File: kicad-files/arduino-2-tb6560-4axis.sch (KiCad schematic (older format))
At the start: 15 parts, among them J1 DB25_Female_MountingHoles, J2 Conn_01x03_Male, J3 Conn_01x02_Male, J4 Conn_01x02_Male, J5 Conn_01x03_Male, J6 Conn_01x02_Male, J7 Conn_01x03_Male, J8 Conn_01x02_Male, J9 Conn_01x02_Male, Q1 2N3904, SW1 SW_Push, SW2 SW_Push

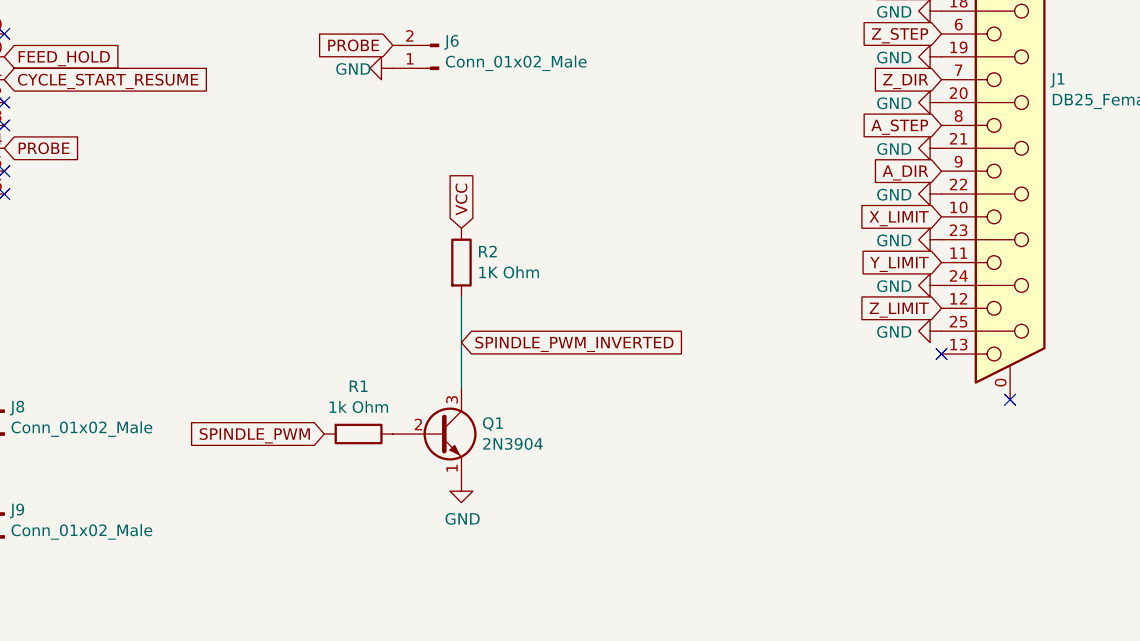
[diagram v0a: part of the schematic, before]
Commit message: more ideas for rev 1.3
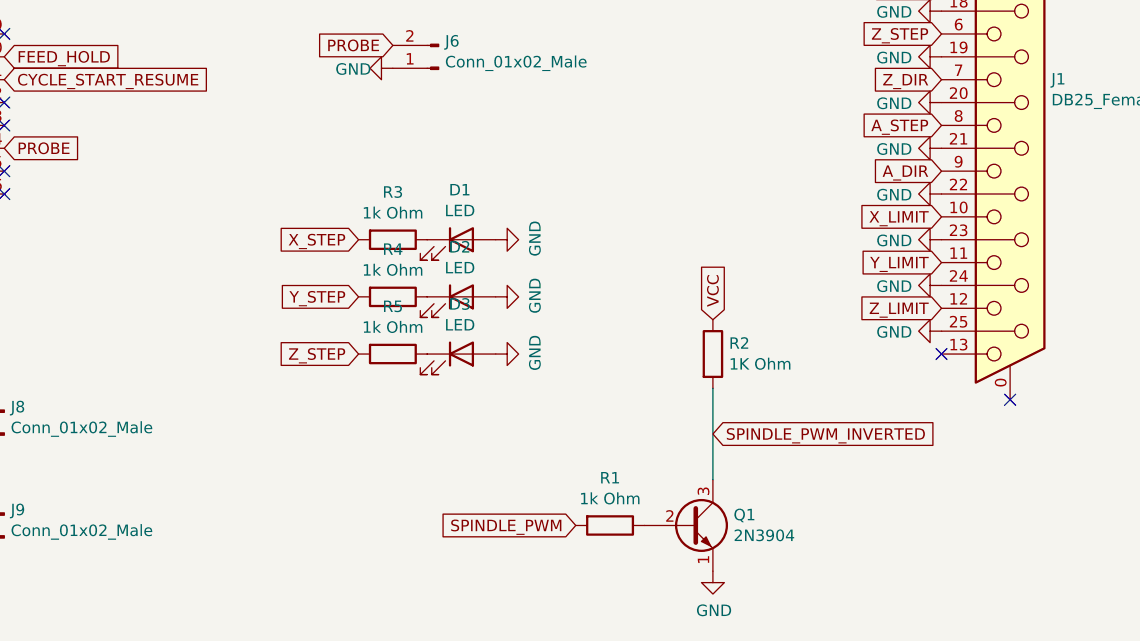
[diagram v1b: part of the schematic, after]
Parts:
- added D1, D2, D3: LED, LED_THT:LED_D5.0mm, symbol Device:LED
- added R3, R4, R5: 1k Ohm, Resistor_THT:R_Axial_DIN0204_L3.6mm_D1.6mm_P5.08mm_Horizontal, symbol Device:R
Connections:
- net GND: now also D1.2 (A), D2.2 (A), D3.2 (A)
- net X_STEP: now also R3.2
- net Y_STEP: now also R4.2
- net Z_STEP: now also R5.2
- new net: D1.1 (K), R3.1
- new net: D2.1 (K), R4.1
- new net: D3.1 (K), R5.1
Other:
- moved on the sheet: Q1, R1, R2
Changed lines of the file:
@@
 L Device:R R1
 U 1 1 5F56F856
-P 5750 5200
-F 0 "R1" V 5543 5200 50  0000 C CNN
-F 1 "1k Ohm" V 5634 5200 50  0000 C CNN
-F 2 "Resistor_THT:R_Axial_DIN0204_L3.6mm_D1.6mm_P5.08mm_Horizontal" V 5680 5200 50  0001 C CNN
-F 3 "~" H 5750 5200 50  0001 C CNN
-	1    5750 5200
+P 6850 5600
+F 0 "R1" V 6643 5600 50  0000 C CNN
+F 1 "1k Ohm" V 6734 5600 50  0000 C CNN
+F 2 "Resistor_THT:R_Axial_DIN0204_L3.6mm_D1.6mm_P5.08mm_Horizontal" V 6780 5600 50  0001 C CNN
+F 3 "~" H 6850 5600 50  0001 C CNN
+	1    6850 5600
 	0    1    1    0
 $EndComp
@@
 L Device:R R2
 U 1 1 5F57191E
-P 6200 4450
-F 0 "R2" H 6270 4496 50  0000 L CNN
-F 1 "1K Ohm" H 6270 4405 50  0000 L CNN
-F 2 "Resistor_THT:R_Axial_DIN0204_L3.6mm_D1.6mm_P5.08mm_Horizontal" V 6130 4450 50  0001 C CNN
-F 3 "~" H 6200 4450 50  0001 C CNN
-	1    6200 4450
+P 7300 4850
+F 0 "R2" H 7370 4896 50  0000 L CNN
+F 1 "1K Ohm" H 7370 4805 50  0000 L CNN
+F 2 "Resistor_THT:R_Axial_DIN0204_L3.6mm_D1.6mm_P5.08mm_Horizontal" V 7230 4850 50  0001 C CNN
+F 3 "~" H 7300 4850 50  0001 C CNN
+	1    7300 4850
 	1    0    0    -1
 $EndComp
@@
 L Transistor_BJT:2N3904 Q1
 U 1 1 5F5721BB
-P 6100 5200
-F 0 "Q1" H 6290 5246 50  0000 L CNN
-F 1 "2N3904" H 6290 5155 50  0000 L CNN
-F 2 "Package_TO_SOT_THT:TO-92_Inline" H 6300 5125 50  0001 L CIN
-F 3 "https://www.fairchildsemi.com/datasheets/2N/2N3904.pdf" H 6100 5200 50  0001 L CNN
-	1    6100 5200
+P 7200 5600
+F 0 "Q1" H 7390 5646 50  0000 L CNN
+F 1 "2N3904" H 7390 5555 50  0000 L CNN
+F 2 "Package_TO_SOT_THT:TO-92_Inline" H 7400 5525 50  0001 L CIN
+F 3 "https://www.fairchildsemi.com/datasheets/2N/2N3904.pdf" H 7200 5600 50  0001 L CNN
+	1    7200 5600
 	1    0    0    -1
 $EndComp
 Text GLabel 3900 2450 1    50   Input ~ 0
 VCC
-Text GLabel 6200 4300 1    50   Input ~ 0
+Text GLabel 7300 4700 1    50   Input ~ 0
 VCC
-Text GLabel 5600 5200 0    50   Input ~ 0
+Text GLabel 6700 5600 0    50   Input ~ 0
 SPINDLE_PWM
 $Comp
 L power:GND #PWR0101
 U 1 1 5F581B0A
-P 6200 5400
-F 0 "#PWR0101" H 6200 5150 50  0001 C CNN
-F 1 "GND" H 6205 5227 50  0000 C CNN
-F 2 "" H 6200 5400 50  0001 C CNN
-F 3 "" H 6200 5400 50  0001 C CNN
-	1    6200 5400
+P 7300 5800
+F 0 "#PWR0101" H 7300 5550 50  0001 C CNN
+F 1 "GND" H 7305 5627 50  0000 C CNN
+F 2 "" H 7300 5800 50  0001 C CNN
+F 3 "" H 7300 5800 50  0001 C CNN
+	1    7300 5800
 	1    0    0    -1
 $EndComp
 Wire Wire Line
-	6200 5000 6200 4600
-Text GLabel 6200 4800 2    50   Input ~ 0
+	7300 5400 7300 5000
+Text GLabel 7300 5200 2    50   Input ~ 0
 SPINDLE_PWM_INVERTED
 Text GLabel 4200 3950 2    50   Input ~ 0
@@
 Text GLabel 4000 5550 0    50   Input ~ 0
 CYCLE_START_RESUME
+$Comp
+L Device:R R3
+U 1 1 5F5D16E5
+P 5900 4350
+F 0 "R3" V 5693 4350 50  0000 C CNN
+F 1 "1k Ohm" V 5784 4350 50  0000 C CNN
+F 2 "Resistor_THT:R_Axial_DIN0204_L3.6mm_D1.6mm_P5.08mm_Horizontal" V 5830 4350 50  0001 C CNN
+F 3 "~" H 5900 4350 50  0001 C CNN
+	1    5900 4350
+	0    1    1    0
+$EndComp
+$Comp
+L Device:R R4
+U 1 1 5F5D1BCB
+P 5900 4600
+F 0 "R4" V 5693 4600 50  0000 C CNN
+F 1 "1k Ohm" V 5784 4600 50  0000 C CNN
+F 2 "Resistor_THT:R_Axial_DIN0204_L3.6mm_D1.6mm_P5.08mm_Horizontal" V 5830 4600 50  0001 C CNN
+F 3 "~" H 5900 4600 50  0001 C CNN
+	1    5900 4600
+	0    1    1    0
+$EndComp
+$Comp
+L Device:R R5
+U 1 1 5F5D1F89
+P 5900 4850
+F 0 "R5" V 5693 4850 50  0000 C CNN
+F 1 "1k Ohm" V 5784 4850 50  0000 C CNN
+F 2 "Resistor_THT:R_Axial_DIN0204_L3.6mm_D1.6mm_P5.08mm_Horizontal" V 5830 4850 50  0001 C CNN
+F 3 "~" H 5900 4850 50  0001 C CNN
+	1    5900 4850
+	0    1    1    0
+$EndComp
+Text GLabel 5750 4350 0    50   Input ~ 0
+X_STEP
+Text GLabel 5750 4600 0    50   Input ~ 0
+Y_STEP
+Text GLabel 5750 4850 0    50   Input ~ 0
+Z_STEP
+$Comp
+L Device:LED D1
+U 1 1 5F5D402B
+P 6200 4350
+F 0 "D1" H 6193 4567 50  0000 C CNN
+F 1 "LED" H 6193 4476 50  0000 C CNN
+F 2 "LED_THT:LED_D5.0mm" H 6200 4350 50  0001 C CNN
+F 3 "~" H 6200 4350 50  0001 C CNN
+	1    6200 4350
+	1    0    0    -1
+$EndComp
+$Comp
+L Device:LED D2
+U 1 1 5F5D6475
+P 6200 4600
+F 0 "D2" H 6193 4817 50  0000 C CNN
+F 1 "LED" H 6193 4726 50  0000 C CNN
+F 2 "LED_THT:LED_D5.0mm" H 6200 4600 50  0001 C CNN
+F 3 "~" H 6200 4600 50  0001 C CNN
+	1    6200 4600
+	1    0    0    -1
+$EndComp
+$Comp
+L Device:LED D3
+U 1 1 5F5D6793
+P 6200 4850
+F 0 "D3" H 6193 5067 50  0000 C CNN
+F 1 "LED" H 6193 4976 50  0000 C CNN
+F 2 "LED_THT:LED_D5.0mm" H 6200 4850 50  0001 C CNN
+F 3 "~" H 6200 4850 50  0001 C CNN
+	1    6200 4850
+	1    0    0    -1
+$EndComp
+$Comp
+L power:GND #PWR0107
+U 1 1 5F5D732B
+P 6350 4350
+F 0 "#PWR0107" H 6350 4100 50  0001 C CNN
+F 1 "GND" H 6355 4177 50  0000 C CNN
+F 2 "" H 6350 4350 50  0001 C CNN
+F 3 "" H 6350 4350 50  0001 C CNN
+	1    6350 4350
+	0    -1   -1   0
+$EndComp
+$Comp
+L power:GND #PWR0108
+U 1 1 5F5D79DB
+P 6350 4600
+F 0 "#PWR0108" H 6350 4350 50  0001 C CNN
+F 1 "GND" H 6355 4427 50  0000 C CNN
+F 2 "" H 6350 4600 50  0001 C CNN
+F 3 "" H 6350 4600 50  0001 C CNN
+	1    6350 4600
+	0    -1   -1   0
+$EndComp
+$Comp
+L power:GND #PWR0109
+U 1 1 5F5D7D83
+P 6350 4850
+F 0 "#PWR0109" H 6350 4600 50  0001 C CNN
+F 1 "GND" H 6355 4677 50  0000 C CNN
+F 2 "" H 6350 4850 50  0001 C CNN
+F 3 "" H 6350 4850 50  0001 C CNN
+	1    6350 4850
+	0    -1   -1   0
+$EndComp
 $EndSCHEMATC
